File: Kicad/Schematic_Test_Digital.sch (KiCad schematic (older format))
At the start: 73 parts, among them J301 JST - 4x1, J302 JST - 4x1, J303 JST - 5x1, J304 JST - 5x1, SW301 RESET PUSH, U301 TSX-3225, U302 LIS3MDLTR, U303 LSM6DS33TR, U304 74HC595PW,112, U305 74HC595PW,112, U306 74HC595PW,112

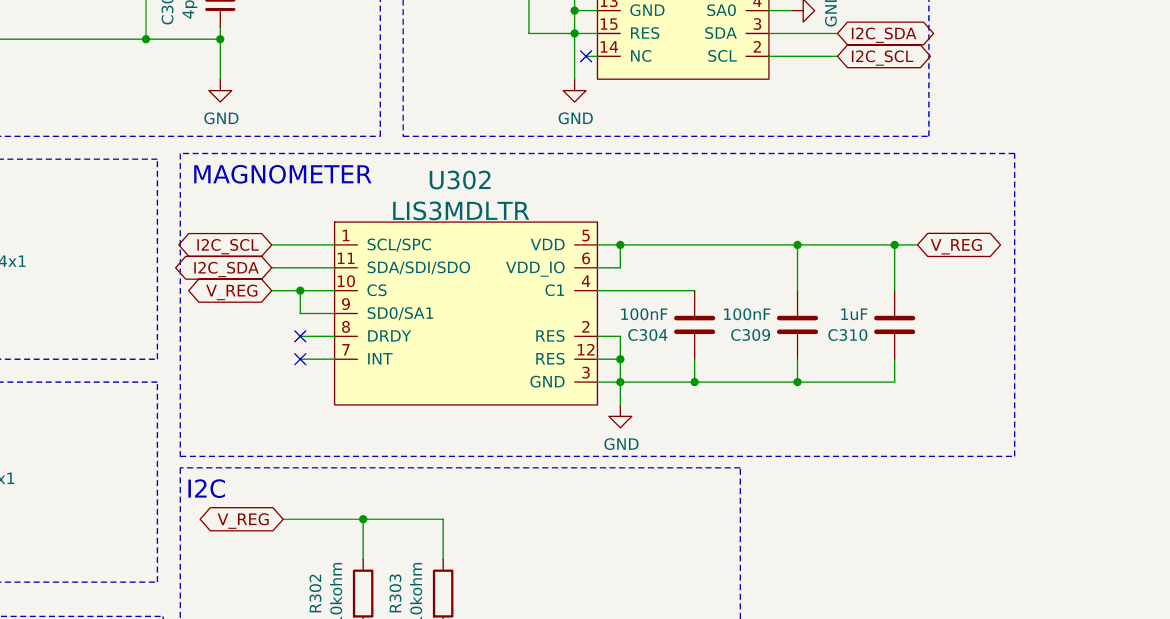
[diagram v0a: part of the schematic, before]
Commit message: Purchases made, case ordered, PCB ordered, parts ordered, money not happy.
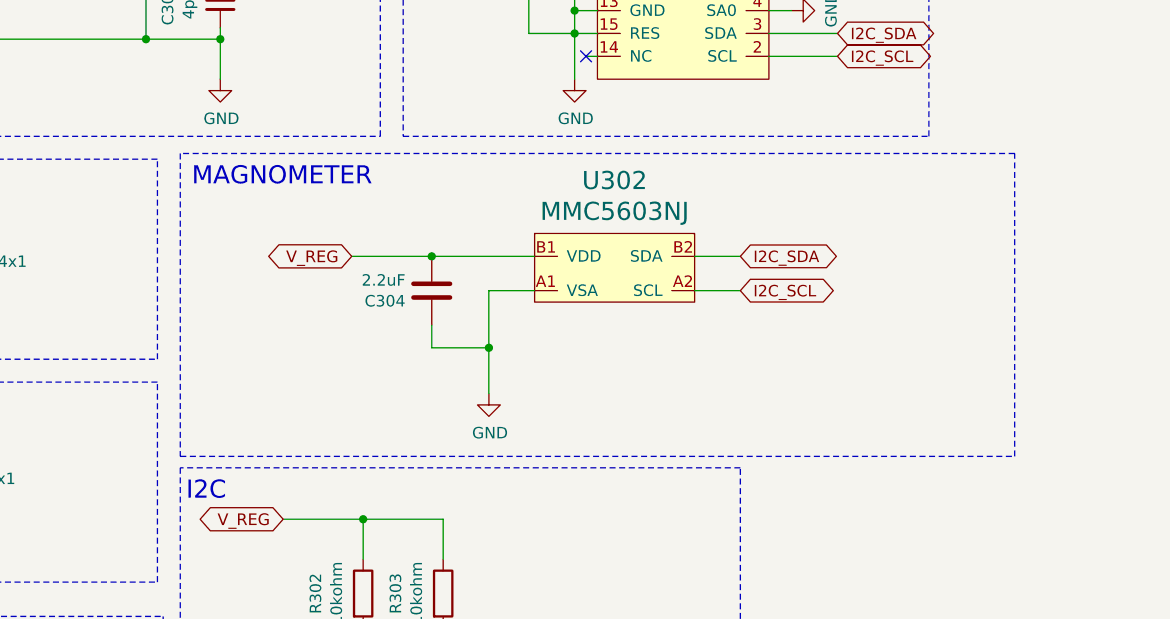
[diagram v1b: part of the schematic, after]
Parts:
- removed C309: 100nF, Capacitor_SMD:C_0805_2012Metric_Pad1.15x1.40mm_HandSolder, symbol Device:C
- removed C310: 1uF, Capacitor_SMD:C_0805_2012Metric_Pad1.15x1.40mm_HandSolder, symbol Device:C
- removed U302: LIS3MDLTR, Package_LGA:LGA-12_2x2mm_P0.5mm, symbol StarGazer:LIS3MDL
- added U302: MMC5603NJ, Kicad:BGA_2_2, symbol StarGazer:MMC5603NJ
- C301, C303: PURCHASED (none) -> 6x IMPORT
- C302: PURCHASED (none) -> 12x
- C304: value 100nF -> 2.2uF; PURCHASED (none) -> 6x
- C305: PURCHASED (none) -> 6x
- C306, C307, C308, U304, U305, U306: PURCHASED (none) -> 9x
- D301, D302, D303, D304, D305, D306, D307, D308, D309, D310, D311, D312, D313, D314, D315, D316, D317, D318, D319, D320, D321, D322, D323, D324: PURCHASED (none) -> 72x
- J301: PURCHASED (none) -> 2x
- J302: PURCHASED (none) -> 5x
- J303: PURCHASED (none) -> 1x
- J304: PURCHASED (none) -> 10x
- R301, R302, R303: PURCHASED (none) -> 24x
- R304, R305, R306, R307, R308, R309, R310, R311, R312, R313, R314, R315, R316, R317, R318, R319, R320, R321, R322, R323, R324, R325, R326, R327: PURCHASED (none) -> 72 (up to 100)
- RV301, SW301, U301, U303: PURCHASED (none) -> 3x
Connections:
- net GND: now also U302.A1 (VSA)
- net I2C_SCL: now also U302.A2 (SCL)
- net I2C_SDA: now also U302.B2 (SDA)
- net V_REG: now also C304.2, U302.B1 (VDD)
- no-connect marks 5 -> 3
